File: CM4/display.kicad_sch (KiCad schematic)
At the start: 1 part, among them U10 4inch_RPi_LCD_(C)

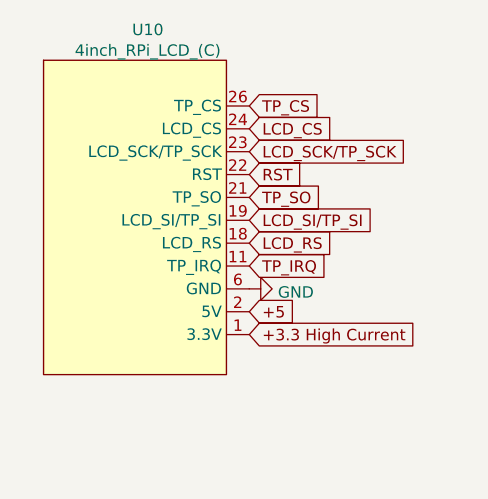
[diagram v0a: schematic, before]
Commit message: Started the "fun" of routing
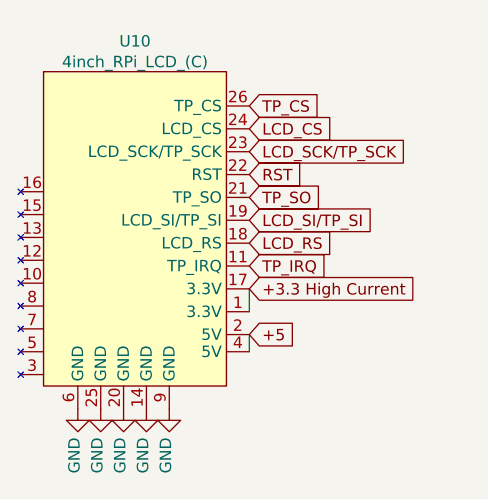
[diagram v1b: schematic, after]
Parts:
- U10: footprint Connector_PinSocket_2.54mm:PinSocket_2x13_P2.54mm_Vertical -> (none)
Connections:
- net +3.3 High Current: now also U10.17 (3.3V)
- net +5: now also U10.4 (5V)
- net GND: now also U10.14 (GND), U10.20 (GND), U10.25 (GND), U10.9 (GND)
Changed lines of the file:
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@@
 (kicad_sch (version 20210126) (generator eeschema)
   (paper "A4")
+  (wire (pts (xy 97.79 107.95) (xy 97.79 110.49))
+    (stroke (width 0) (type solid) (color 0 0 0 0))
+  )
+  (wire (pts (xy 97.79 113.03) (xy 97.79 114.935))
+    (stroke (width 0) (type solid) (color 0 0 0 0))
+  )
   (global_label "TP_CS" (shape input) (at 97.79 87.63 0)
     (effects (font (size 1.27 1.27)) (justify left))
@@
     )
   )
-  (global_label "+5" (shape input) (at 97.79 110.49 0)
+  (global_label "+3.3 High Current" (shape input) (at 97.79 107.95 0)
     (effects (font (size 1.27 1.27)) (justify left))
-    (property "Intersheet References" "${INTERSHEET_REFS}" (id 0) (at 102.985 110.4106 0)
+    (property "Intersheet References" "${INTERSHEET_REFS}" (id 0) (at 117.9226 107.8706 0)
       (effects (font (size 1.27 1.27)) (justify left) hide)
     )
   )
-  (global_label "+3.3 High Current" (shape input) (at 97.79 113.03 0)
+  (global_label "+5" (shape input) (at 97.79 113.03 0)
     (effects (font (size 1.27 1.27)) (justify left))
-    (property "Intersheet References" "${INTERSHEET_REFS}" (id 0) (at 117.9226 112.9506 0)
+    (property "Intersheet References" "${INTERSHEET_REFS}" (id 0) (at 102.985 112.9506 0)
       (effects (font (size 1.27 1.27)) (justify left) hide)
     )
   )
-  (symbol (lib_id "power:GND") (at 97.79 107.95 90) (unit 1)
+  (symbol (lib_id "power:GND") (at 78.74 121.285 0) (unit 1)
     (in_bom yes) (on_board yes)
-    (property "Reference" "#PWR0148" (id 0) (at 104.14 107.95 0)
+    (property "Reference" "#PWR0152" (id 0) (at 78.74 127.635 0)
       (effects (font (size 1.27 1.27)) hide)
     )
-    (property "Value" "GND" (id 1) (at 100.9651 108.3385 90)
+    (property "Value" "GND" (id 1) (at 78.3515 124.4601 90)
       (effects (font (size 1.27 1.27)) (justify right))
     )
-    (property "Footprint" "" (id 2) (at 97.79 107.95 0)
+    (property "Footprint" "" (id 2) (at 78.74 121.285 0)
       (effects (font (size 1.27 1.27)) hide)
     )
-    (property "Datasheet" "" (id 3) (at 97.79 107.95 0)
+    (property "Datasheet" "" (id 3) (at 78.74 121.285 0)
       (effects (font (size 1.27 1.27)) hide)
     )
     (pin "1")
   )
-  (symbol (lib_id "teensy:4inch_RPi_LCD_(C)") (at 85.725 101.6 0) (unit 1)
+  (symbol (lib_id "power:GND") (at 81.28 121.285 0) (unit 1)
     (in_bom yes) (on_board yes)
-    (property "Reference" "U10" (id 0) (at 86.5124 79.1676 0))
-    (property "Value" "4inch_RPi_LCD_(C)" (id 1) (at 86.5124 81.4663 0))
-    (property "Footprint" "Connector_PinSocket_2.54mm:PinSocket_2x13_P2.54mm_Vertical" (id 2) (at 85.09 45.085 0)
+    (property "Reference" "#PWR0151" (id 0) (at 81.28 127.635 0)
       (effects (font (size 1.27 1.27)) hide)
     )
-    (property "Datasheet" "" (id 3) (at 85.09 45.085 0)
+    (property "Value" "GND" (id 1) (at 80.8915 124.4601 90)
+      (effects (font (size 1.27 1.27)) (justify right))
+    )
+    (property "Footprint" "" (id 2) (at 81.28 121.285 0)
+      (effects (font (size 1.27 1.27)) hide)
+    )
+    (property "Datasheet" "" (id 3) (at 81.28 121.285 0)
       (effects (font (size 1.27 1.27)) hide)
     )
     (pin "1")
+  )
+  (symbol (lib_id "power:GND") (at 83.82 121.285 0) (unit 1)
+    (in_bom yes) (on_board yes)
+    (property "Reference" "#PWR0150" (id 0) (at 83.82 127.635 0)
+      (effects (font (size 1.27 1.27)) hide)
+    )
+    (property "Value" "GND" (id 1) (at 83.4315 124.4601 90)
+      (effects (font (size 1.27 1.27)) (justify right))
+    )
+    (property "Footprint" "" (id 2) (at 83.82 121.285 0)
+      (effects (font (size 1.27 1.27)) hide)
+    )
+    (property "Datasheet" "" (id 3) (at 83.82 121.285 0)
+      (effects (font (size 1.27 1.27)) hide)
+    )
+    (pin "1")
+  )
+  (symbol (lib_id "power:GND") (at 86.36 121.285 0) (unit 1)
+    (in_bom yes) (on_board yes)
+    (property "Reference" "#PWR0149" (id 0) (at 86.36 127.635 0)
+      (effects (font (size 1.27 1.27)) hide)
+    )
+    (property "Value" "GND" (id 1) (at 85.9715 124.4601 90)
+      (effects (font (size 1.27 1.27)) (justify right))
+    )
+    (property "Footprint" "" (id 2) (at 86.36 121.285 0)
+      (effects (font (size 1.27 1.27)) hide)
+    )
+    (property "Datasheet" "" (id 3) (at 86.36 121.285 0)
+      (effects (font (size 1.27 1.27)) hide)
+    )
+    (pin "1")
+  )
+  (symbol (lib_id "power:GND") (at 88.9 121.285 0) (unit 1)
+    (in_bom yes) (on_board yes)
+    (property "Reference" "#PWR0148" (id 0) (at 88.9 127.635 0)
+      (effects (font (size 1.27 1.27)) hide)
+    )
+    (property "Value" "GND" (id 1) (at 88.5115 124.4601 90)
+      (effects (font (size 1.27 1.27)) (justify right))
+    )
+    (property "Footprint" "" (id 2) (at 88.9 121.285 0)
+      (effects (font (size 1.27 1.27)) hide)
+    )
+    (property "Datasheet" "" (id 3) (at 88.9 121.285 0)
+      (effects (font (size 1.27 1.27)) hide)
+    )
+    (pin "1")
+  )
+  (symbol (lib_id "teensy:4inch_RPi_LCD_(C)") (at 25.4 105.41 0) (unit 1)
+    (in_bom yes) (on_board yes)
+    (property "Reference" "U10" (id 0) (at 85.09 80.4376 0))
+    (property "Value" "4inch_RPi_LCD_(C)" (id 1) (at 85.09 82.7363 0))
+    (property "Footprint" "" (id 2) (at 24.765 48.895 0)
+      (effects (font (size 1.27 1.27)) hide)
+    )
+    (property "Datasheet" "" (id 3) (at 24.765 48.895 0)
+      (effects (font (size 1.27 1.27)) hide)
+    )
+    (pin "1")
+    (pin "10")
     (pin "11")
+    (pin "12")
+    (pin "13")
+    (pin "14")
+    (pin "15")
+    (pin "16")
+    (pin "17")
     (pin "18")
     (pin "19")
     (pin "2")
+    (pin "20")
     (pin "21")
     (pin "22")
     (pin "23")
     (pin "24")
+    (pin "25")
     (pin "26")
+    (pin "3")
+    (pin "4")
+    (pin "5")
     (pin "6")
+    (pin "7")
+    (pin "8")
+    (pin "9")
   )
 )
